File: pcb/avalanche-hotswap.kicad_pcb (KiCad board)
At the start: 2 copper layers, 158 x 126.6 mm, 138 parts, among them J1 TRRS, J2 OLED, P1 i2c_pin, P2 i2c_pin, P3 battery+, P4 battery-, SW0 SW_Push, SW1 SW_Push, SW10 SW_Push, SW11 SW_Push, SW12 SW_Push, SW13 SW_Push, SW14 SW_Push, SW15 SW_Push, SW16 SW_Push, SW17 SW_Push, SW18 SW_Push, SW19 SW_Push, SW2 SW_Push, SW20 SW_Push, SW21 SW_Push, SW22 SW_Push, SW23 SW_Push, SW24 SW_Push, SW25 SW_Push, SW26 SW_Push, SW27 SW_Push, SW28 SW_Push, SW29 SW_Push, SW3 SW_Push, SW30 SW_Push, SW31 SW_Push, SW32 SW_Push, SW33 SW_DPDT_x2, SW34 SW_DPDT_x2, SW4 SW_Push, SW5 SW_Push, SW6 SW_Push, SW7 SW_Push, SW8 SW_Push, SW9 SW_Push, U1 ProMicro

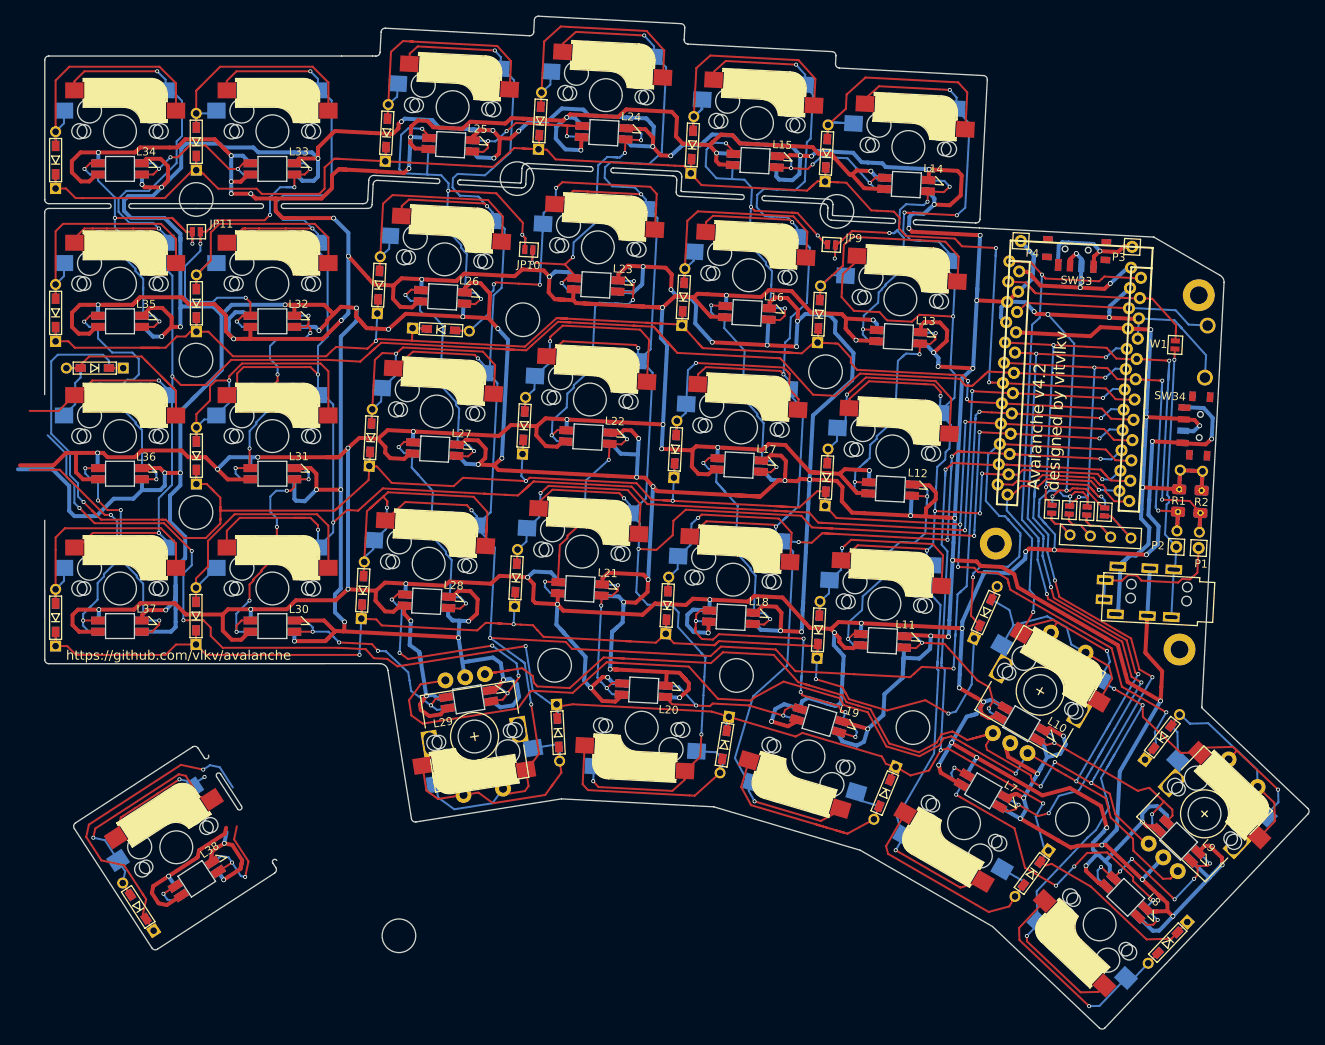
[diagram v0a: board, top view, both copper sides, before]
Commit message: Final changes of palm release.
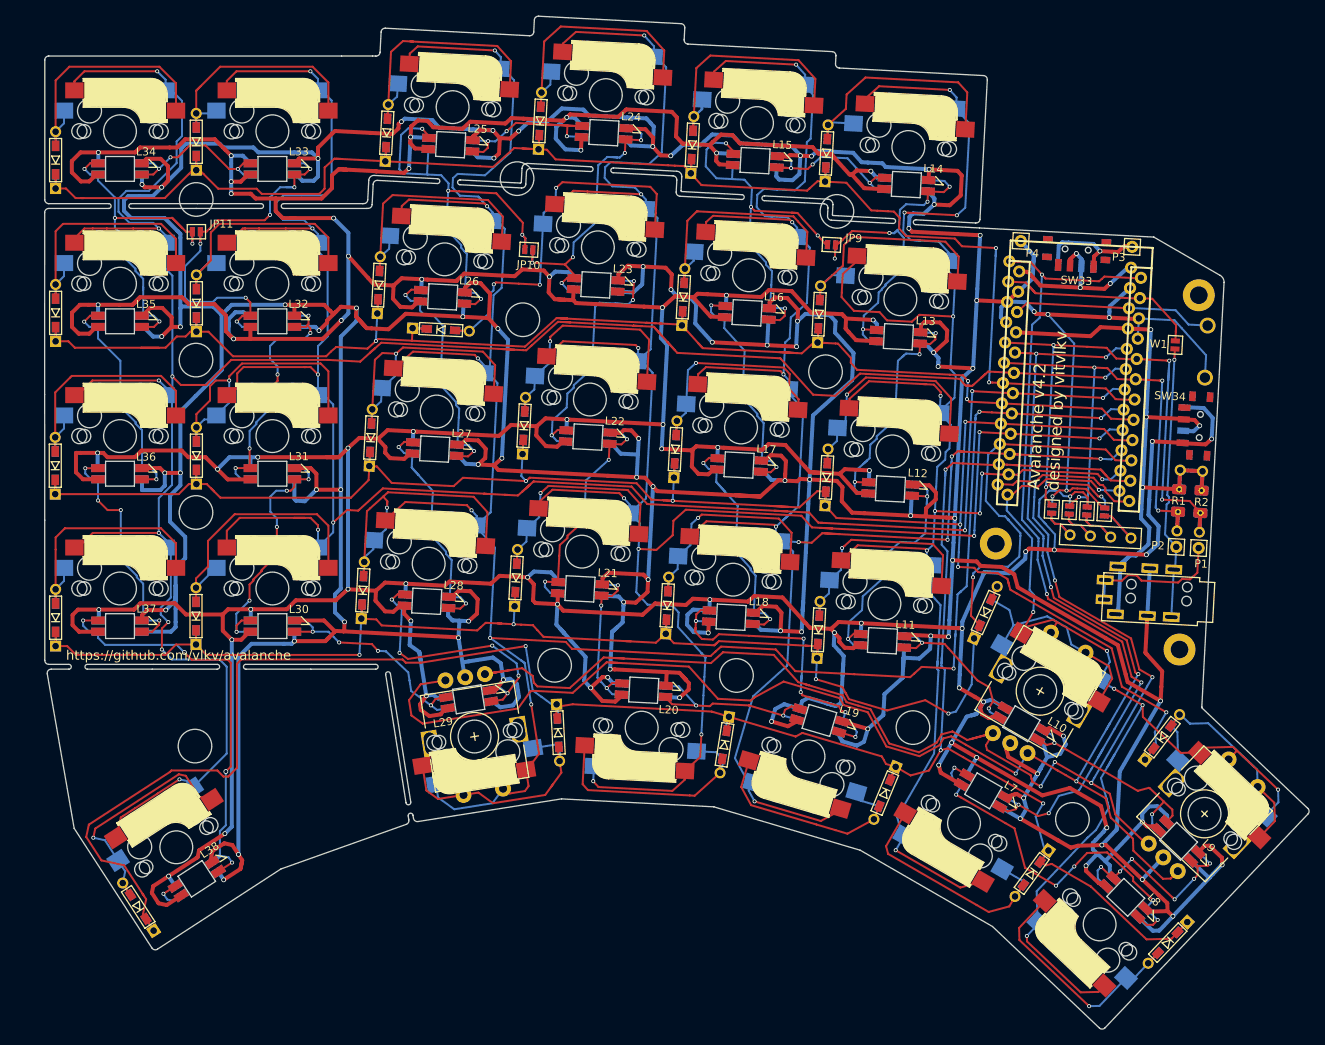
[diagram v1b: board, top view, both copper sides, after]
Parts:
- moved HM5 34.8 mm to (99.4, 117.0)
- moved D13 13.2 mm to (81.9, 81.9), turned to 90 degrees
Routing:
- net row2: track 273.0 -> 237.5 mm, vias 7 -> 6
- net row4: track 309.6 -> 276.8 mm, vias 8 -> 4
- net col0: track 286.7 -> 318.8 mm, vias 8 -> 9
- net Net-(L37-Pad2): track 47.7 -> 54.4 mm
- net Net-(D22-Pad2): track 44.7 -> 40.1 mm
- net GND: track 1153.8 -> 1158.1 mm, vias 78 -> 77
- net Net-(L35-Pad2): track 32.4 -> 28.6 mm
- net Net-(D30-Pad2): track 32.9 -> 29.5 mm
- net Net-(D6-Pad2): track 35.8 -> 32.7 mm
- net VCC: track 973.3 -> 976.3 mm
- net row0: track 195.4 -> 192.8 mm
- net Net-(D10-Pad2): track 49.2 -> 47.1 mm
- net Net-(D2-Pad2): track 33.1 -> 32.0 mm
- net Net-(D7-Pad2): track 33.7 -> 32.6 mm
- net Net-(D1-Pad2): track 34.2 -> 33.1 mm
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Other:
- outline, holes or cut-outs redrawn
- net class Default removed
